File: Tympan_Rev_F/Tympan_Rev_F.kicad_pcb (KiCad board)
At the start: 4 copper layers, 38 x 74 mm, 91 parts, among them IC1 BC127, J1 SJ-3523-SMT-TR, J2 SJ-3524-SMT-TR-PI, J3 Conn_01x06, J4 Qwiik Connector, P1 CONN_01X06, P2 CONN_01X06, P3 CONN_01X06, P4 CONN_01X06, P6 CONN_01X01, P7 CONN_01X01, P8 CONN_01X01, SW1 CL-SB-22A, SW2 SW_Push, U1 MCP73831, U2 TLV320AIC3206IRSBT, U3 74LVC1G66, U4 LP5907MFX-1.8, U5 Teensy4.1, U6 LC709203

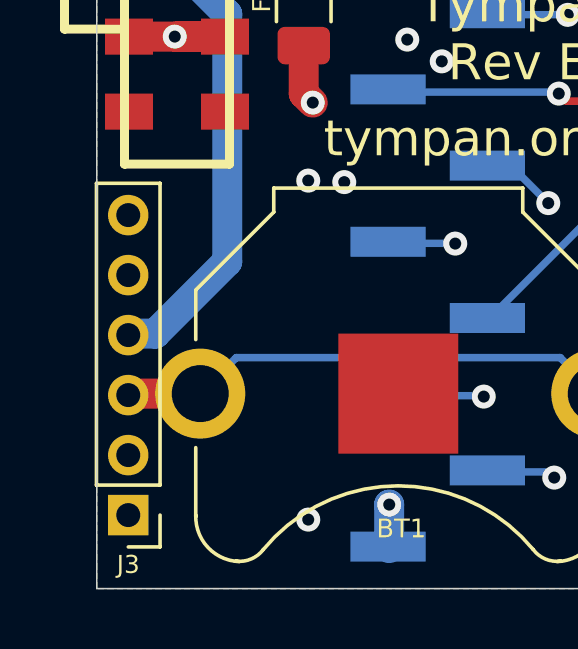
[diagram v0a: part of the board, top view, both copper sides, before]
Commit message: minor edit save
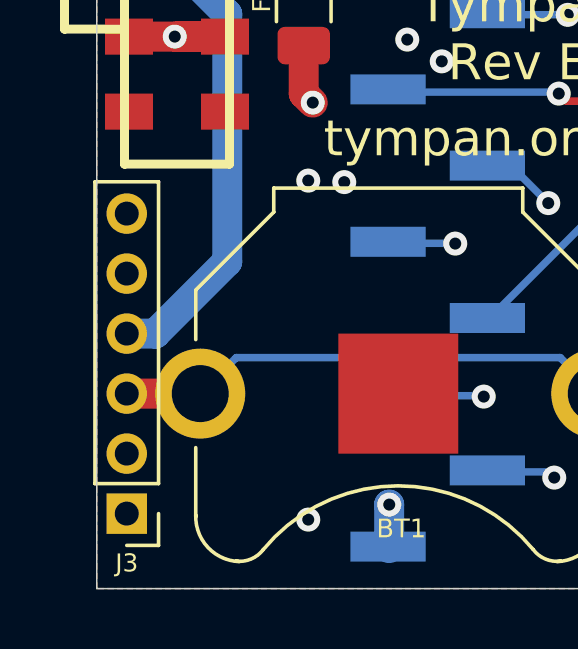
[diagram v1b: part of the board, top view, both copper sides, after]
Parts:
- moved J3 0.07 mm to (135.4, 130.7)
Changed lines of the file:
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@@
   )
   (footprint "Pin_Headers:Pin_Header_Straight_1x06_Pitch2.00mm" (layer "F.Cu")
-    (at 135.45 130.75 180)
+    (at 135.4 130.7 180)
     (descr "Through hole straight pin header, 1x06, 2.00mm pitch, single row")
     (tags "Through hole pin header THT 1x06 2.00mm single row")
@@
   (segment (start 142.65 128.1) (end 142.65 119.65) (width 0.25) (layer "In2.Cu") (net 135))
   (segment (start 164.375001 105.051999) (end 164.375001 114.624999) (width 0.25) (layer "In2.Cu") (net 135))
-  (segment (start 135.45 130.75) (end 140 130.75) (width 0.25) (layer "In2.Cu") (net 135))
+  (segment (start 135.4 130.7) (end 139.95 130.7) (width 0.25) (layer "In2.Cu") (net 135))
   (segment (start 162.65 78.47) (end 164.98 78.47) (width 0.25) (layer "B.Cu") (net 135))
   (segment (start 164.98 78.47) (end 165 78.45) (width 0.25) (layer "B.Cu") (net 135))
